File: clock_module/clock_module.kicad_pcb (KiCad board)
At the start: 4 copper layers, 70 x 34 mm, 41 parts, among them J1 Connector, USB-TYPE-C-16P, J2 Conn_01x03, SW1 SW_SPDT, U1 USBLC6-2SC6, U2 NE555DR, U3 NE555DR, U4 74HC08D, U5 74HC32D, U6 NE555DR, U7 74HC04D

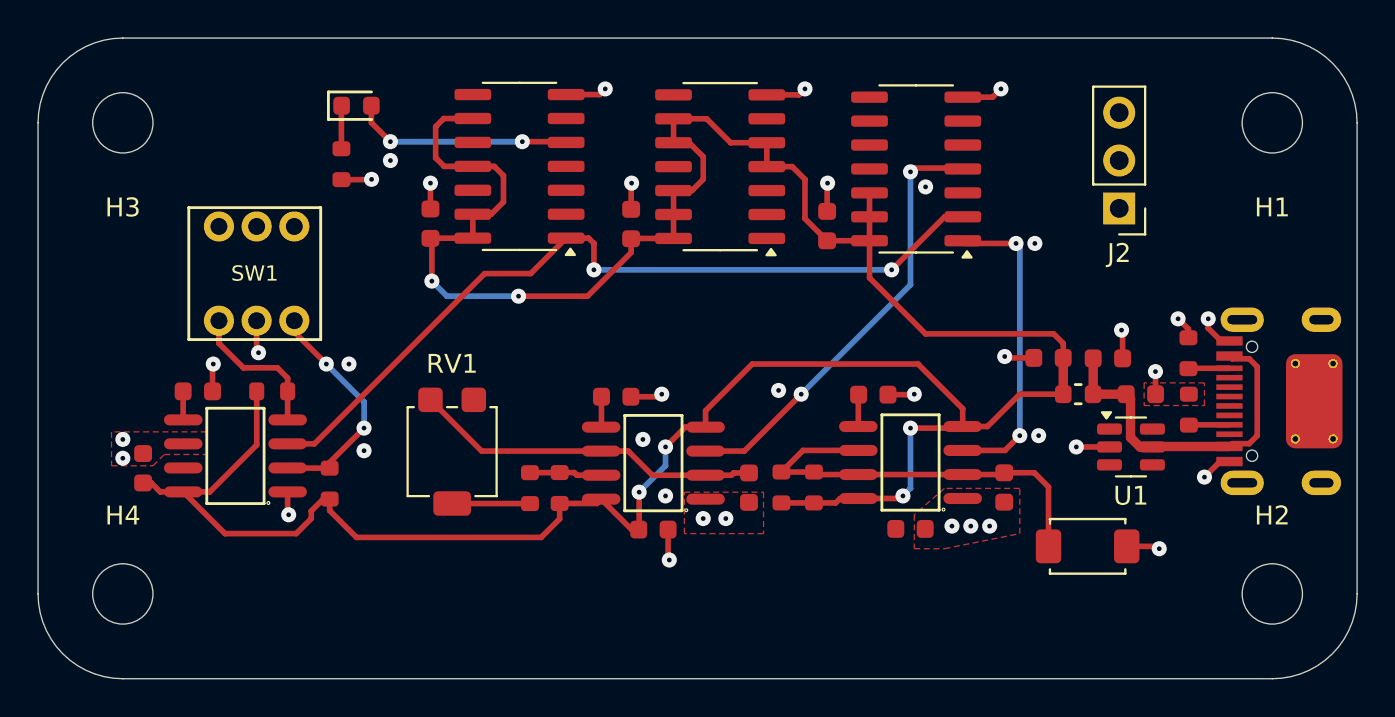
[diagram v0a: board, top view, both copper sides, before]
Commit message: finished board
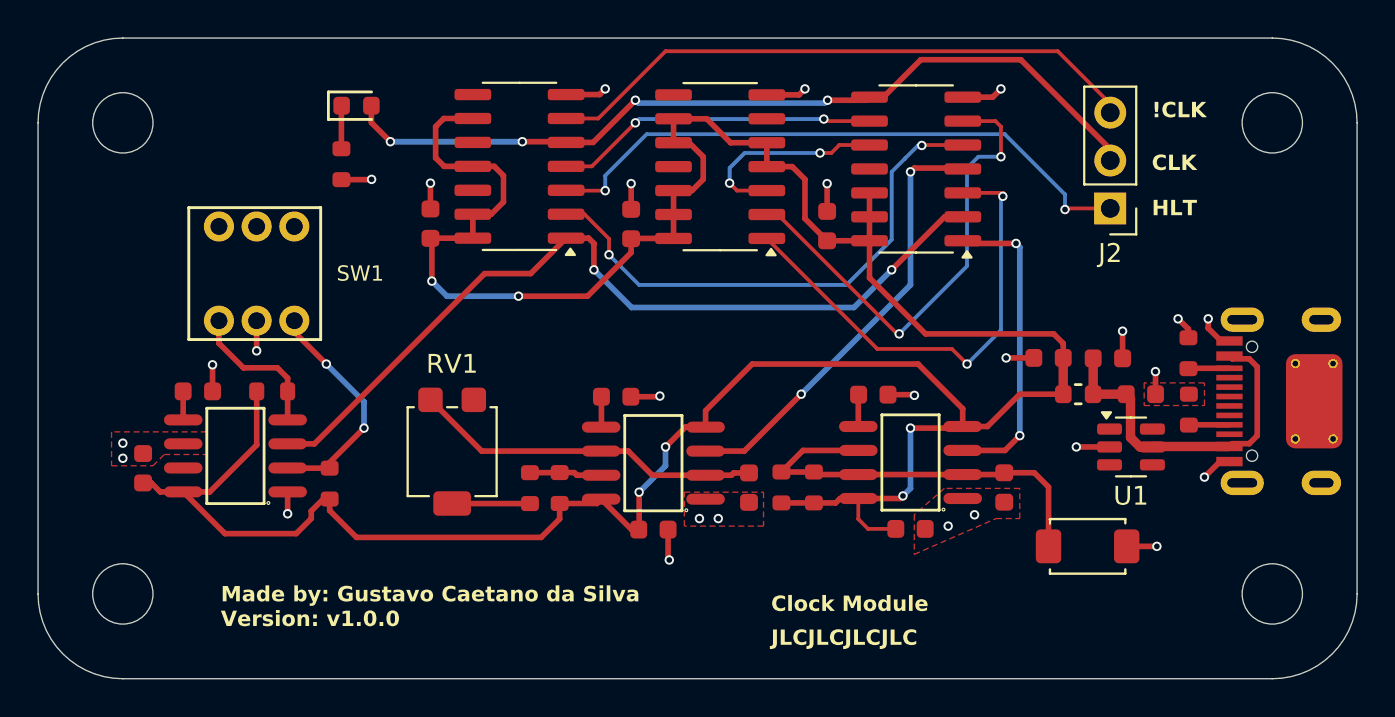
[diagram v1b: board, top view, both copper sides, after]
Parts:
- moved J2 0.47 mm to (154.4, 66.5)
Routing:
- net /Main Circuit/CLK_SIGNAL: track 11.7 -> 45.3 mm, vias 2 -> 4
- net /Main Circuit/HLT: track 0.00 -> 33.2 mm, vias 0 -> 2
- net /Main Circuit/!CLK_SIGNAL: track 0.00 -> 32.2 mm
- net /Main Circuit/!SIG_SELECT: track 0.00 -> 28.3 mm, vias 0 -> 2
- net Net-(U4-2Y): track 0.00 -> 25.7 mm, vias 0 -> 2
- net Net-(U4-1Y): track 0.00 -> 25.5 mm, vias 0 -> 2
- net Net-(U4-3A): track 0.00 -> 17.2 mm, vias 0 -> 2
- net Net-(U4-3B): track 0.00 -> 10.9 mm, vias 0 -> 2
- net +5V: track 158.1 -> 161.4 mm
- net /Main Circuit/SIG_SELECT: track 43.0 -> 44.7 mm
- net GND: track 34.4 -> 33.6 mm, vias 37 -> 27
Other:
- board text added: "!CLK"
- board text added: "CLK"
- board text added: "Clock Module"
- board text added: "HLT"
- board text added: "JLCJLCJLCJLC"
- board text added: "Made by: Gustavo Caetano da Silva Version: v1.0.0"
